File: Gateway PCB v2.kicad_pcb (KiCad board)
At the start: 4 copper layers, 83.2 x 39.5 mm, 109 parts, among them J1 Conn_Coaxial, J2 Conn_01x04_Pin, J3 Conn_02x03_Odd_Even, J4 Conn_01x03_Pin, U6 TPS7A91, U7 TLV62568ADRL, X1 TG2016SMN 32.0000M-TCGNNMB

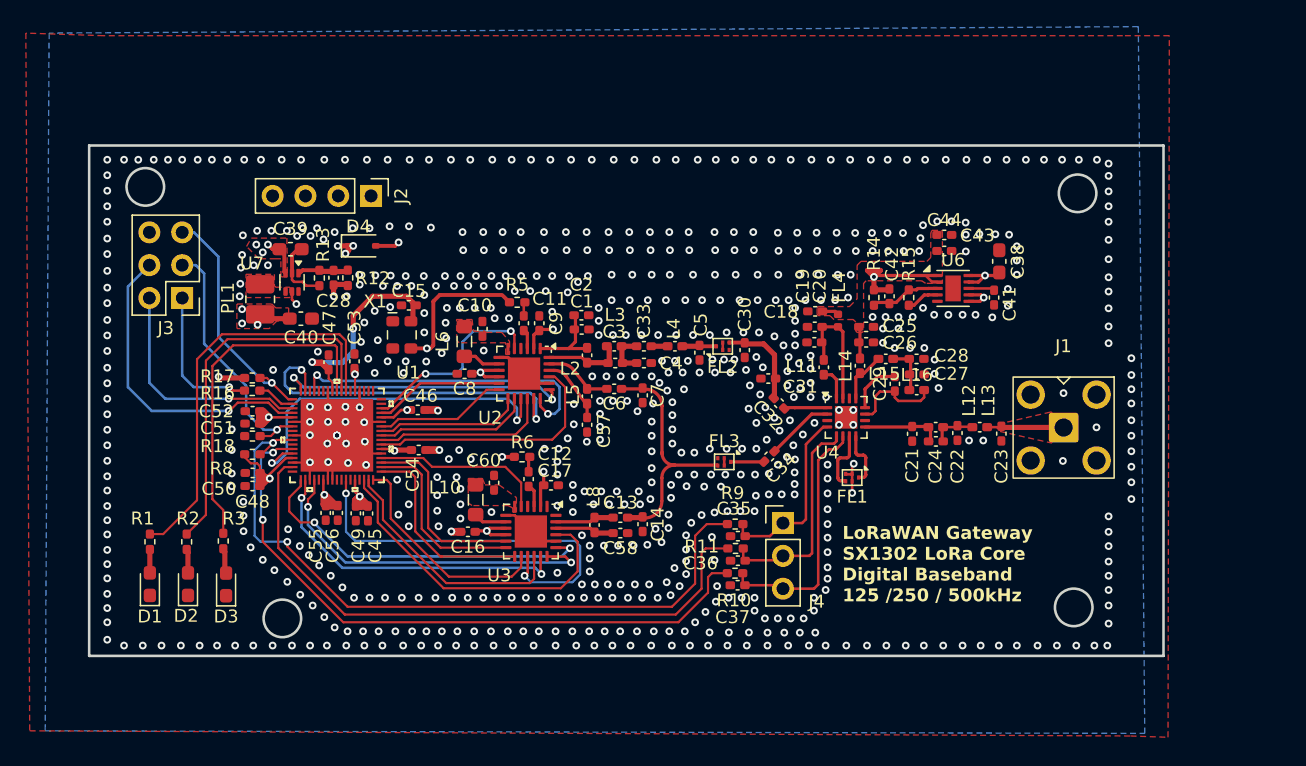
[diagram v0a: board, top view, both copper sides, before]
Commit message: UpDate
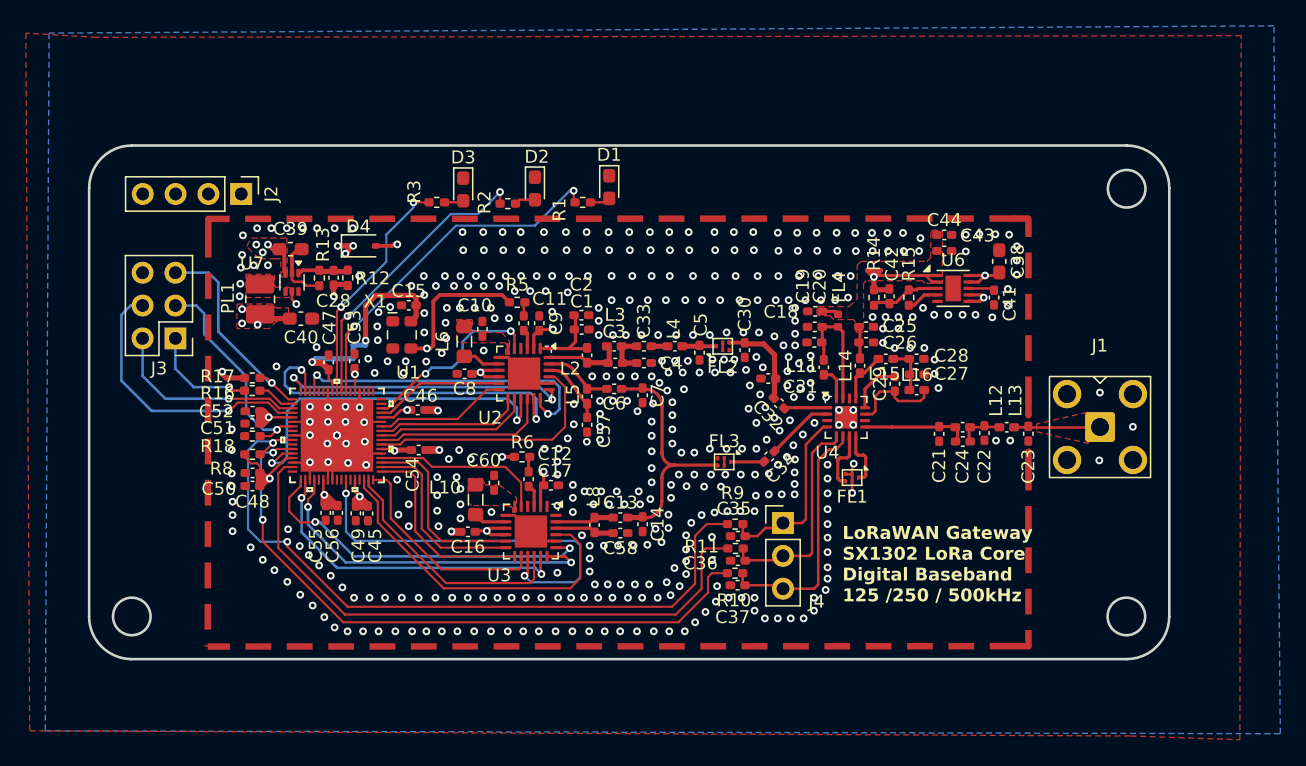
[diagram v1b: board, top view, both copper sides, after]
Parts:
- added NT1: NetTie_2, NetTie:NetTie-2_SMD_Pad0.5mm, F.Cu at (86.5, 85.1)
- added NT2: NetTie_2, NetTie:NetTie-2_SMD_Pad0.5mm, F.Cu at (86.5, 88.9)
- added NT3: NetTie_2, NetTie:NetTie-2_SMD_Pad0.5mm, F.Cu at (86.0, 70.3)
- added NT4: NetTie_2, NetTie:NetTie-2_SMD_Pad0.5mm, F.Cu at (23.0, 70.9)
- added NT5: NetTie_2, NetTie:NetTie-2_SMD_Pad0.5mm, F.Cu at (86.0, 103.5)
- moved D1 47.0 mm to (54.0, 67.9), turned to -90 degrees
- moved R1 42.6 mm to (52.0, 69.1), turned to 0 degrees
- moved D2 40.7 mm to (48.3, 68.0), turned to -90 degrees
- moved R2 36.1 mm to (46.2, 69.2), turned to 0 degrees
- moved D3 35.7 mm to (42.8, 68.1), turned to -90 degrees
- moved R3 31.0 mm to (40.7, 69.1), turned to 0 degrees
- moved J2 10.1 mm to (25.6, 68.5)
- moved J3 3.17 mm to (20.5, 79.6)
- moved J1 2.82 mm to (92.0, 86.5)
- moved C21 2.09 mm to (79.6, 87.0)
- moved C22 2.09 mm to (83.1, 87.0)
- moved C24 2.09 mm to (81.4, 87.6)
- moved L12 2.09 mm to (81.4, 86.5)
- moved C23 2.09 mm to (86.5, 87.0)
- moved L13 2.09 mm to (84.8, 86.5)
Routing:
- net Net-(U1-GPIO[3]): track 27.1 -> 18.3 mm, vias 0 -> 2
- net Net-(U1-GPIO[4]): track 29.0 -> 22.9 mm, vias 0 -> 2
- net GND2: track 0.00 -> 5.00 mm
- net Net-(U1-GPIO[5]): track 32.1 -> 27.6 mm, vias 0 -> 2
- net 3.3V: track 94.4 -> 98.5 mm
- net EX_HOST_MISO: track 11.3 -> 8.40 mm
- net EX_HOST_MOSI: track 18.5 -> 15.6 mm
- net EX_HOST_RESET: track 20.0 -> 17.3 mm
- net EX_HOST_SCK: track 24.2 -> 21.8 mm
- net 5V: track 17.3 -> 19.6 mm
- net EX_HOST_CSN: track 18.6 -> 16.4 mm
- net Net-(U4-ANT): track 6.20 -> 8.29 mm
- net Net-(J1-In): track 6.15 -> 7.01 mm
- net SX1302_CSD: track 55.2 -> 56.0 mm
- net RADIO_B_IQ_3: track 26.1 -> 26.7 mm
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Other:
- board size 83.2 x 39.5 mm -> 83.6 x 39.8 mm
